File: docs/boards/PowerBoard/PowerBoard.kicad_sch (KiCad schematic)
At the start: 0 parts

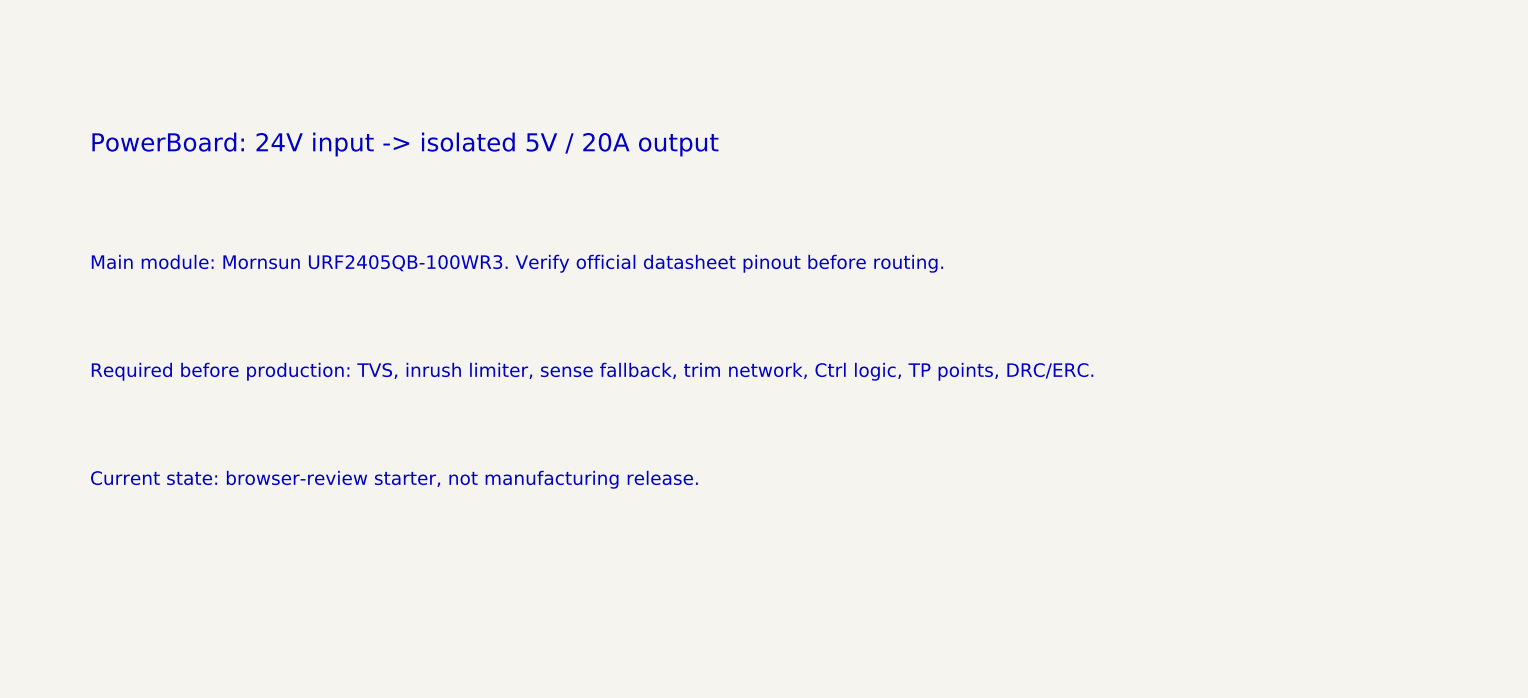
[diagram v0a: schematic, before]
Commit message: v4F generate real PowerBoard schematic from netlist lock
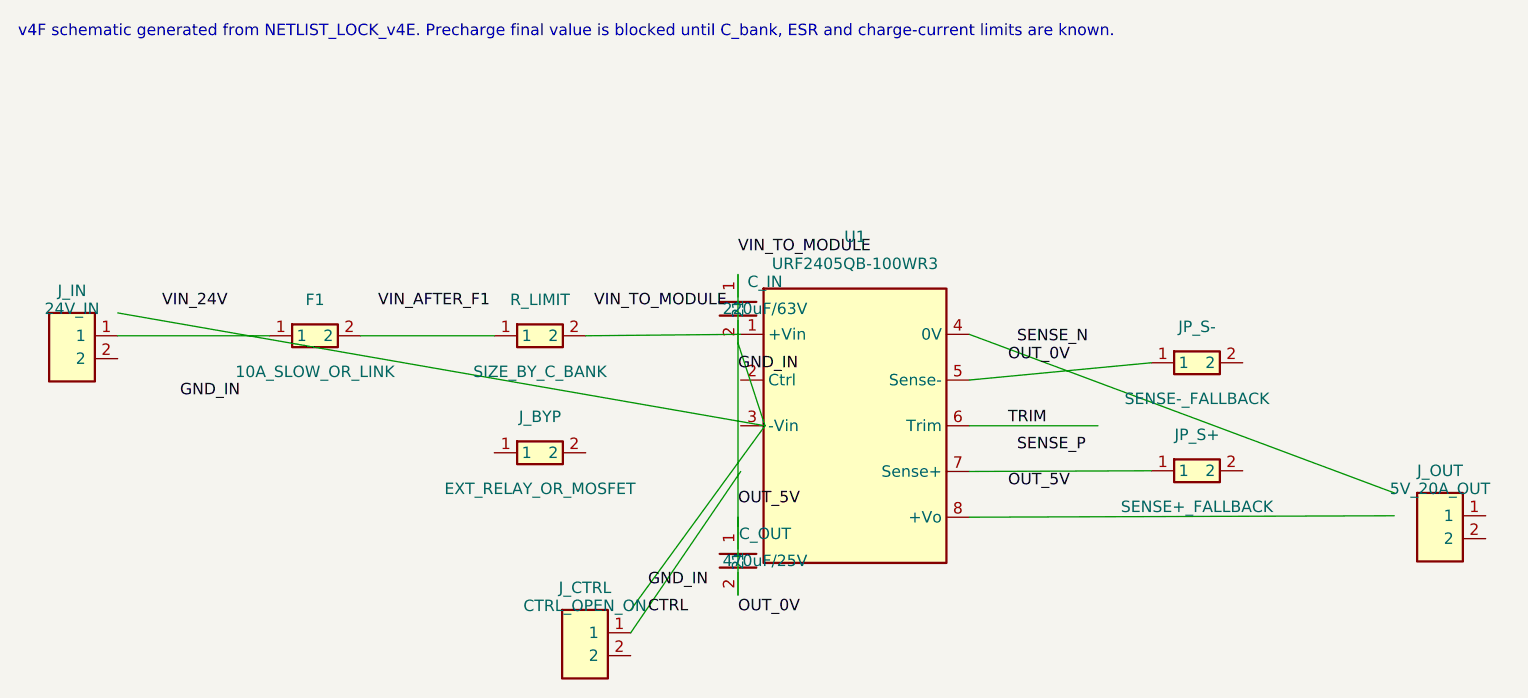
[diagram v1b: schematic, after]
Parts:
- added C_IN: 220uF/63V, CP_Radial, symbol Custom:CAP2
- added C_OUT: 470uF/25V, CP_Radial, symbol Custom:CAP2
- added F1: 10A_SLOW_OR_LINK, Fuse_or_Link_10A, symbol Custom:PASSIVE_2P
- added JP_S+: SENSE+_FALLBACK, Sense_Jumper_Plus, symbol Custom:PASSIVE_2P
- added JP_S-: SENSE-_FALLBACK, Sense_Jumper_Minus, symbol Custom:PASSIVE_2P
- added J_BYP: EXT_RELAY_OR_MOSFET, External_Bypass_Header, symbol Custom:PASSIVE_2P
- added J_CTRL: CTRL_OPEN_ON, Header_1x2, symbol Custom:CONN_2P
- added J_IN: 24V_IN, Terminal_IN_2P, symbol Custom:CONN_2P
- added J_OUT: 5V_20A_OUT, Terminal_OUT_2P_30A, symbol Custom:CONN_2P
- added R_LIMIT: SIZE_BY_C_BANK, Precharge_R, symbol Custom:PASSIVE_2P
- added U1: URF2405QB-100WR3, Mornsun_URF2405QB_100WR3_QB, symbol Custom:URF_QB
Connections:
- new net: F1.1, J_IN.1
- new net: F1.2, R_LIMIT.1
- new net: R_LIMIT.2, U1.1 (+Vin)
- new net: JP_S-.1, U1.5 (Sense-)
- new net: JP_S+.1, U1.7 (Sense+)
- new net GND_IN: C_IN.1, C_OUT.1, C_OUT.2
- new net TRIM: U1.6 (Trim)
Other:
- note added: "v4F schematic generated from NETLIST_LOCK_v4E. Precharge final value is blocked until C_bank, ESR and charge-current limits are known."
- note removed: "Current state: browser-review starter, not manufacturing release."
- note removed: "Main module: Mornsun URF2405QB-100WR3. Verify official datasheet pinout before routing."
- note removed: "PowerBoard: 24V input -> isolated 5V / 20A output"
- note removed: "Required before production: TVS, inrush limiter, sense fallback, trim network, Ctrl logic, TP points, DRC/ERC."
- title: PowerBoard starter -> PowerBoard
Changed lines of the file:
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@@
 (kicad_sch (version 20230121) (generator "eeschema")
-  (paper "A4")
-  (title_block (title "PowerBoard starter") (date "2026-06-14") (rev "v3-starter") (company "Docreate Mod"))
-  (text "PowerBoard: 24V input -> isolated 5V / 20A output" (at 20 25 0) (effects (font (size 2 2) (thickness 0.25)) (justify left bottom)))
-  (text "Main module: Mornsun URF2405QB-100WR3. Verify official datasheet pinout before routing." (at 20 38 0) (effects (font (size 1.5 1.5) (thickness 0.2)) (justify left bottom)))
-  (text "Required before production: TVS, inrush limiter, sense fallback, trim network, Ctrl logic, TP points, DRC/ERC." (at 20 50 0) (effects (font (size 1.5 1.5) (thickness 0.2)) (justify left bottom)))
-  (text "Current state: browser-review starter, not manufacturing release." (at 20 62 0) (effects (font (size 1.5 1.5) (thickness 0.2)) (justify left bottom)))
+  (paper "A3")
+  (title_block (title "PowerBoard") (date "2026-06-14") (rev "v4F") (company "Docreate Mod"))
+  (text "v4F schematic generated from NETLIST_LOCK_v4E. Precharge final value is blocked until C_bank, ESR and charge-current limits are known." (at 12 12 0) (effects (font (size 1.27 1.27) (thickness 0.18)) (justify left bottom)))
+  (symbol (lib_id "Custom:CONN_2P") (at 18 45 0) (unit 1) (in_bom yes) (on_board yes) (dnp no)
+    (property "Reference" "J_IN" (at 18 40 0) (effects (font (size 1.27 1.27))))
+    (property "Value" "24V_IN" (at 18 42 0) (effects (font (size 1.27 1.27))))
+    (property "Footprint" "Terminal_IN_2P" (at 18 45 0) (effects (font (size 1.27 1.27)) hide))
+    (pin "1")
+    (pin "2")
+  )
+  (symbol (lib_id "Custom:PASSIVE_2P") (at 45 45 0) (unit 1) (in_bom yes) (on_board yes) (dnp no)
+    (property "Reference" "F1" (at 45 41 0) (effects (font (size 1.27 1.27))))
+    (property "Value" "10A_SLOW_OR_LINK" (at 45 49 0) (effects (font (size 1.27 1.27))))
+    (property "Footprint" "Fuse_or_Link_10A" (at 45 45 0) (effects (font (size 1.27 1.27)) hide))
+    (pin "1")
+    (pin "2")
+  )
+  (symbol (lib_id "Custom:PASSIVE_2P") (at 70 45 0) (unit 1) (in_bom yes) (on_board yes) (dnp no)
+    (property "Reference" "R_LIMIT" (at 70 41 0) (effects (font (size 1.27 1.27))))
+    (property "Value" "SIZE_BY_C_BANK" (at 70 49 0) (effects (font (size 1.27 1.27))))
+    (property "Footprint" "Precharge_R" (at 70 45 0) (effects (font (size 1.27 1.27)) hide))
+    (pin "1")
+    (pin "2")
+  )
+  (symbol (lib_id "Custom:PASSIVE_2P") (at 70 58 0) (unit 1) (in_bom yes) (on_board yes) (dnp no)
+    (property "Reference" "J_BYP" (at 70 54 0) (effects (font (size 1.27 1.27))))
+    (property "Value" "EXT_RELAY_OR_MOSFET" (at 70 62 0) (effects (font (size 1.27 1.27))))
+    (property "Footprint" "External_Bypass_Header" (at 70 58 0) (effects (font (size 1.27 1.27)) hide))
+    (pin "1")
+    (pin "2")
+  )
+  (symbol (lib_id "Custom:URF_QB") (at 105 55 0) (unit 1) (in_bom yes) (on_board yes) (dnp no)
+    (property "Reference" "U1" (at 105 34 0) (effects (font (size 1.27 1.27))))
+    (property "Value" "URF2405QB-100WR3" (at 105 37 0) (effects (font (size 1.27 1.27))))
+    (property "Footprint" "Mornsun_URF2405QB_100WR3_QB" (at 105 55 0) (effects (font (size 1.27 1.27)) hide))
+    (pin "1")
+    (pin "2")
+    (pin "3")
+    (pin "4")
+    (pin "5")
+    (pin "6")
+    (pin "7")
+    (pin "8")
+  )
+  (symbol (lib_id "Custom:CAP2") (at 92 42 0) (unit 1) (in_bom yes) (on_board yes) (dnp no)
+    (property "Reference" "C_IN" (at 95 39 0) (effects (font (size 1.27 1.27))))
+    (property "Value" "220uF/63V" (at 95 42 0) (effects (font (size 1.27 1.27))))
+    (property "Footprint" "CP_Radial" (at 92 42 0) (effects (font (size 1.27 1.27)) hide))
+    (pin "1")
+    (pin "2")
+  )
+  (symbol (lib_id "Custom:CAP2") (at 92 70 0) (unit 1) (in_bom yes) (on_board yes) (dnp no)
+    (property "Reference" "C_OUT" (at 95 67 0) (effects (font (size 1.27 1.27))))
+    (property "Value" "470uF/25V" (at 95 70 0) (effects (font (size 1.27 1.27))))
+    (property "Footprint" "CP_Radial" (at 92 70 0) (effects (font (size 1.27 1.27)) hide))
+    (pin "1")
+    (pin "2")
+  )
+  (symbol (lib_id "Custom:PASSIVE_2P") (at 143 60 0) (unit 1) (in_bom yes) (on_board yes) (dnp no)
+    (property "Reference" "JP_S+" (at 143 56 0) (effects (font (size 1.27 1.27))))
+    (property "Value" "SENSE+_FALLBACK" (at 143 64 0) (effects (font (size 1.27 1.27))))
+    (property "Footprint" "Sense_Jumper_Plus" (at 143 60 0) (effects (font (size 1.27 1.27)) hide))
+    (pin "1")
+    (pin "2")
+  )
+  (symbol (lib_id "Custom:PASSIVE_2P") (at 143 48 0) (unit 1) (in_bom yes) (on_board yes) (dnp no)
+    (property "Reference" "JP_S-" (at 143 44 0) (effects (font (size 1.27 1.27))))
+    (property "Value" "SENSE-_FALLBACK" (at 143 52 0) (effects (font (size 1.27 1.27))))
+    (property "Footprint" "Sense_Jumper_Minus" (at 143 48 0) (effects (font (size 1.27 1.27)) hide))
+    (pin "1")
+    (pin "2")
+  )
+  (symbol (lib_id "Custom:CONN_2P") (at 170 65 0) (unit 1) (in_bom yes) (on_board yes) (dnp no)
+    (property "Reference" "J_OUT" (at 170 60 0) (effects (font (size 1.27 1.27))))
+    (property "Value" "5V_20A_OUT" (at 170 62 0) (effects (font (size 1.27 1.27))))
+    (property "Footprint" "Terminal_OUT_2P_30A" (at 170 65 0) (effects (font (size 1.27 1.27)) hide))
+    (pin "1")
+    (pin "2")
+  )
+  (symbol (lib_id "Custom:CONN_2P") (at 75 78 0) (unit 1) (in_bom yes) (on_board yes) (dnp no)
+    (property "Reference" "J_CTRL" (at 75 73 0) (effects (font (size 1.27 1.27))))
+    (property "Value" "CTRL_OPEN_ON" (at 75 75 0) (effects (font (size 1.27 1.27))))
+    (property "Footprint" "Header_1x2" (at 75 78 0) (effects (font (size 1.27 1.27)) hide))
+    (pin "1")
+    (pin "2")
+  )
+  (wire (pts (xy 23.08 45) (xy 39.92 45)) (stroke (width 0) (type default)))
+  (label "VIN_24V" (at 28 42 0) (effects (font (size 1.27 1.27)) (justify left bottom)))
+  (wire (pts (xy 23.08 42.46) (xy 95 55)) (stroke (width 0) (type default)))
+  (label "GND_IN" (at 30 52 0) (effects (font (size 1.27 1.27)) (justify left bottom)))
+  (wire (pts (xy 50.08 45) (xy 64.92 45)) (stroke (width 0) (type default)))
+  (label "VIN_AFTER_F1" (at 52 42 0) (effects (font (size 1.27 1.27)) (justify left bottom)))
+  (wire (pts (xy 75.08 45) (xy 92.3 44.84)) (stroke (width 0) (type default)))
+  (label "VIN_TO_MODULE" (at 76 42 0) (effects (font (size 1.27 1.27)) (justify left bottom)))
+  (wire (pts (xy 92 38.19) (xy 92 44.84)) (stroke (width 0) (type default)))
+  (label "VIN_TO_MODULE" (at 92 36 0) (effects (font (size 1.27 1.27)) (justify left bottom)))
+  (wire (pts (xy 92 45.81) (xy 95 55)) (stroke (width 0) (type default)))
+  (label "GND_IN" (at 92 49 0) (effects (font (size 1.27 1.27)) (justify left bottom)))
+  (wire (pts (xy 117.7 65.16) (xy 164.92 65)) (stroke (width 0) (type default)))
+  (label "OUT_5V" (at 122 62 0) (effects (font (size 1.27 1.27)) (justify left bottom)))
+  (wire (pts (xy 117.7 44.84) (xy 164.92 62.46)) (stroke (width 0) (type default)))
+  (label "OUT_0V" (at 122 48 0) (effects (font (size 1.27 1.27)) (justify left bottom)))
+  (wire (pts (xy 117.7 49.92) (xy 137.92 48)) (stroke (width 0) (type default)))
+  (label "SENSE_N" (at 123 46 0) (effects (font (size 1.27 1.27)) (justify left bottom)))
+  (wire (pts (xy 117.7 55) (xy 132 55)) (stroke (width 0) (type default)))
+  (label "TRIM" (at 122 55 0) (effects (font (size 1.27 1.27)) (justify left bottom)))
+  (wire (pts (xy 117.7 60.08) (xy 137.92 60)) (stroke (width 0) (type default)))
+  (label "SENSE_P" (at 123 58 0) (effects (font (size 1.27 1.27)) (justify left bottom)))
+  (wire (pts (xy 92 66.19) (xy 92 65.16)) (stroke (width 0) (type default)))
+  (label "OUT_5V" (at 92 64 0) (effects (font (size 1.27 1.27)) (justify left bottom)))
+  (wire (pts (xy 92 73.81) (xy 92 44.84)) (stroke (width 0) (type default)))
+  (label "OUT_0V" (at 92 76 0) (effects (font (size 1.27 1.27)) (justify left bottom)))
+  (wire (pts (xy 80.08 78) (xy 92.3 60.08)) (stroke (width 0) (type default)))
+  (label "CTRL" (at 82 76 0) (effects (font (size 1.27 1.27)) (justify left bottom)))
+  (wire (pts (xy 80.08 75.46) (xy 95 55)) (stroke (width 0) (type default)))
+  (label "GND_IN" (at 82 73 0) (effects (font (size 1.27 1.27)) (justify left bottom)))
   (sheet_instances (path "/" (page "1")))
 )
